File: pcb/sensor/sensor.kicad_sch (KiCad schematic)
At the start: 18 parts, among them J11 adc_sensor2, J12 adc_sensor1, J3 can_sensor, SW1 SW_SPST, U1 HX711, U2 SIT1042AQT/3, U9 HX711

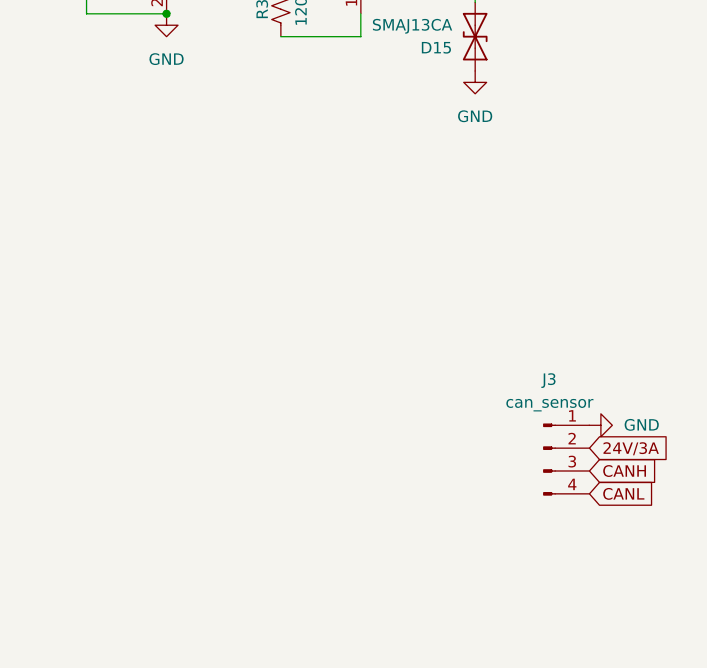
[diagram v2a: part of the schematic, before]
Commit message: feat: update
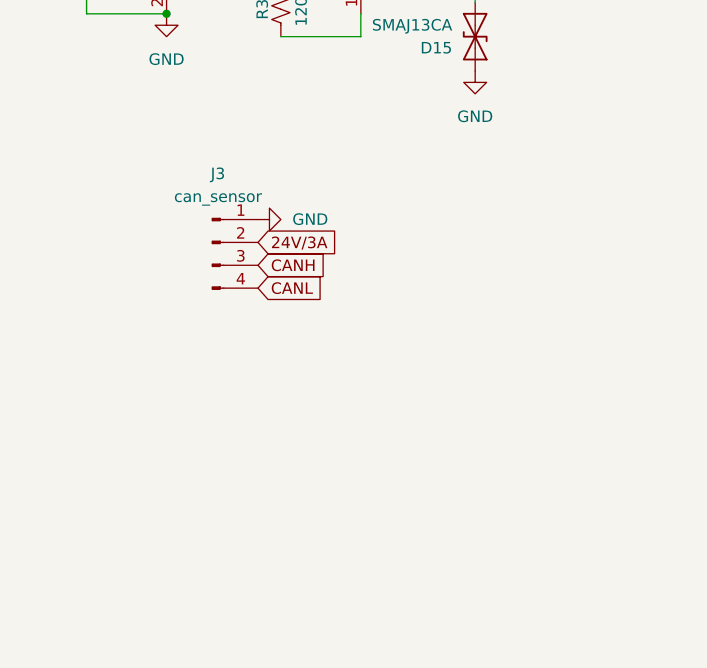
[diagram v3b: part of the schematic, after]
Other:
- moved on the sheet: J3
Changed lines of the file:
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@@
 	(global_label "CANH"
 		(shape input)
-		(at 250.19 129.54 0)
+		(at 213.36 106.68 0)
 		(fields_autoplaced yes)
 		(effects
@@
 		)
 		(property "Intersheetrefs" "${INTERSHEET_REFS}"
-			(at 258.1948 129.54 0)
+			(at 221.3648 106.68 0)
 			(hide yes)
 			(effects
@@
 	(global_label "24V{slash}3A"
 		(shape input)
-		(at 250.19 127 0)
+		(at 213.36 104.14 0)
 		(fields_autoplaced yes)
 		(effects
@@
 		)
 		(property "Intersheetrefs" "${INTERSHEET_REFS}"
-			(at 260.3114 127 0)
+			(at 223.4814 104.14 0)
 			(hide yes)
 			(effects
@@
 	(global_label "CANL"
 		(shape input)
-		(at 250.19 132.08 0)
+		(at 213.36 109.22 0)
 		(fields_autoplaced yes)
 		(effects
@@
 		)
 		(property "Intersheetrefs" "${INTERSHEET_REFS}"
-			(at 257.8924 132.08 0)
+			(at 221.0624 109.22 0)
 			(hide yes)
 			(effects
@@
 	(symbol
 		(lib_id "power:GND")
-		(at 250.19 124.46 90)
+		(at 213.36 101.6 90)
 		(unit 1)
 		(exclude_from_sim no)
@@
 		(fields_autoplaced yes)
 		(property "Reference" "#PWR062"
-			(at 256.54 124.46 0)
+			(at 219.71 101.6 0)
 			(hide yes)
 			(effects
@@
 		)
 		(property "Value" "GND"
-			(at 254 124.4601 90)
+			(at 217.17 101.6001 90)
 			(effects
 				(font
@@
 		)
 		(property "Footprint" ""
-			(at 250.19 124.46 0)
+			(at 213.36 101.6 0)
 			(hide yes)
 			(effects
@@
 		)
 		(property "Datasheet" ""
-			(at 250.19 124.46 0)
+			(at 213.36 101.6 0)
 			(hide yes)
 			(effects
@@
 		)
 		(property "Description" "Power symbol creates a global label with name \"GND\" , ground"
-			(at 250.19 124.46 0)
+			(at 213.36 101.6 0)
 			(hide yes)
 			(effects
@@
 	(symbol
 		(lib_id "Connector:Conn_01x04_Pin")
-		(at 245.11 127 0)
+		(at 208.28 104.14 0)
 		(unit 1)
 		(exclude_from_sim no)
@@
 		(fields_autoplaced yes)
 		(property "Reference" "J3"
-			(at 245.745 119.38 0)
+			(at 208.915 96.52 0)
 			(effects
 				(font
@@
 		)
 		(property "Value" "can_sensor"
-			(at 245.745 121.92 0)
+			(at 208.915 99.06 0)
 			(effects
 				(font
@@
 		)
 		(property "Footprint" "Connector_JST:JST_PH_B4B-PH-K_1x04_P2.00mm_Vertical"
-			(at 245.11 127 0)
+			(at 208.28 104.14 0)
 			(hide yes)
 			(effects
@@
 		)
 		(property "Datasheet" "~"
-			(at 245.11 127 0)
+			(at 208.28 104.14 0)
 			(hide yes)
 			(effects
@@
 		)
 		(property "Description" "Generic connector, single row, 01x04, script generated"
-			(at 245.11 127 0)
-			(hide yes)
-			(effects
+			(at 208.28 104.14 0)
+			(hide yes)
+			(effects

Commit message: feat: update
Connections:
- net GND: now also U2.9 (EP)
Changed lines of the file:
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@@
 		)
 		(property "Footprint" "Package_DFN_QFN:DFN-8-1EP_3x3mm_P0.65mm_EP1.5x2.25mm"
-			(at 203.2 68.58 0)
+			(at 202.946 73.152 0)
 			(hide yes)
 			(effects
